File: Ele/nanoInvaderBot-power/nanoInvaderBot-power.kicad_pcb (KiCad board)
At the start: 2 copper layers, 72 x 40 mm, 16 parts, among them J1 S6B-ZR-SM4A-TF(LF)(SN), J2 S6B-ZR-SM4A-TF(LF)(SN), J3 1746142-1, J4 Conn_01x20, P1 USB_C_Plug_USB2.0, U4 BQ25170DSGR, U5 TLV61048DBVT

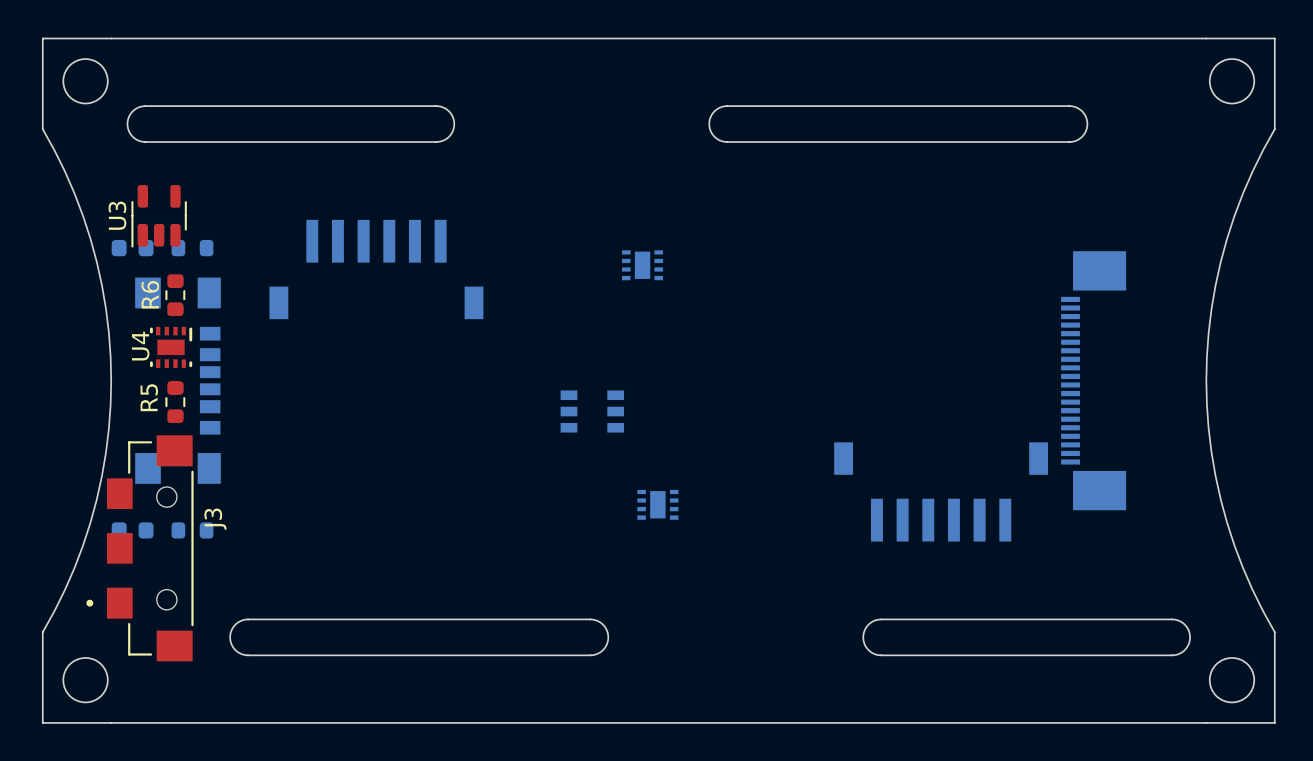
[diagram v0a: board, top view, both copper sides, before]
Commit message: Intermediate state -power layer almost done
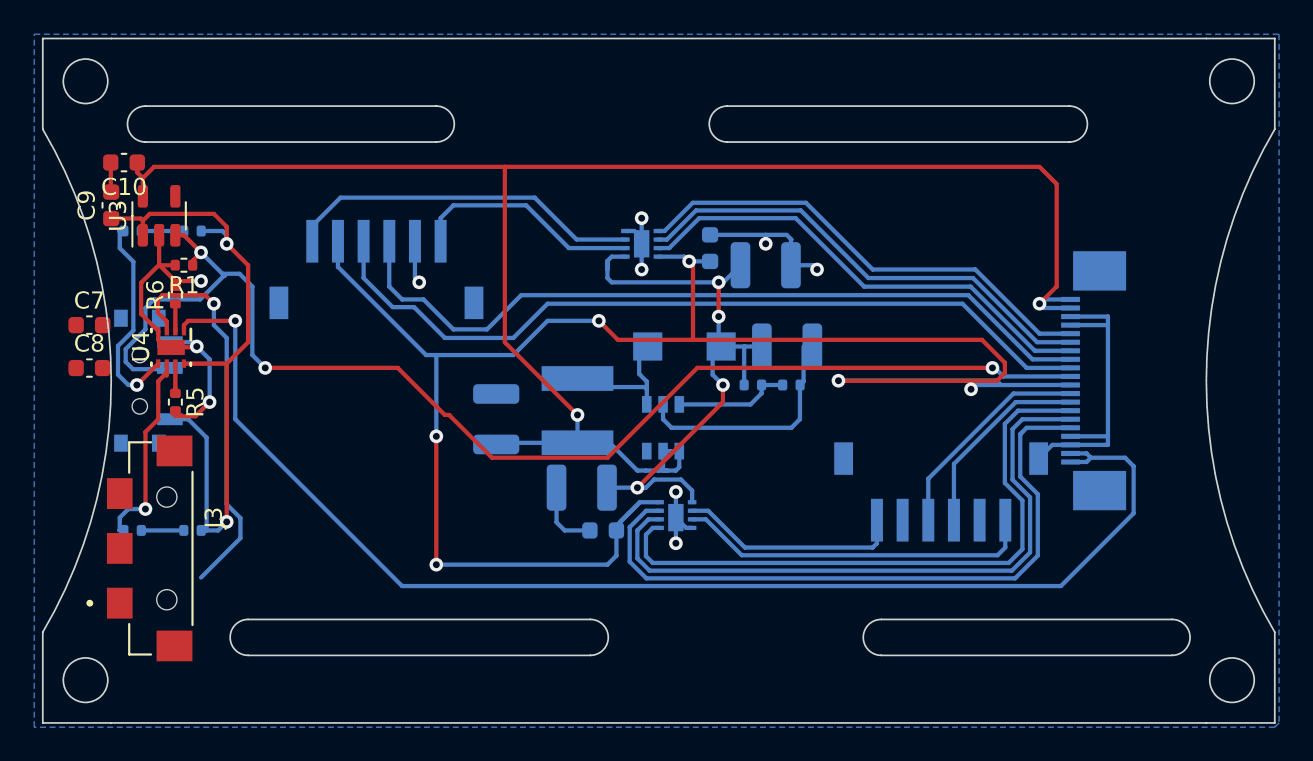
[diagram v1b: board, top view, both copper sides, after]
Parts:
- removed P1: USB_C_Plug_USB2.0, Connector_USB:USB_C_Receptacle_GCT_USB4135-GF-A_6P_TopMnt_Horizontal
- added C1: C, Capacitor_SMD:C_1210_3225Metric, B.Cu at (140.5, 102.2)
- added C10: C, Capacitor_SMD:C_0603_1608Metric, F.Cu at (118.8, 87.2)
- added C2: C, Capacitor_SMD:C_1210_3225Metric, B.Cu at (157.5, 98.0)
- added C3: C, Capacitor_SMD:C_1210_3225Metric, B.Cu at (156.2, 93.2)
- added C4: C, Capacitor_SMD:C_0603_1608Metric, B.Cu at (153.0, 92.2)
- added C5: C, Capacitor_SMD:C_1210_3225Metric, B.Cu at (145.5, 106.2)
- added C6: C, Capacitor_SMD:C_0603_1608Metric, B.Cu at (146.8, 108.8)
- added C7: C, Capacitor_SMD:C_0603_1608Metric, F.Cu at (116.7, 96.8)
- added C8: C, Capacitor_SMD:C_0603_1608Metric, F.Cu at (116.7, 99.3)
- added C9: C, Capacitor_SMD:C_0603_1608Metric, F.Cu at (118.0, 89.8)
- added D3: D, footprints:SDO_B120AF_DIO, B.Cu at (151.5, 98.0)
- added L1: L, footprints:IND_SWPA5040S_SNL, B.Cu at (145.2, 101.8)
- added R1: R, Resistor_SMD:R_0402_1005Metric, F.Cu at (122.2, 93.2)
- added R10: R, Resistor_SMD:R_0402_1005Metric, B.Cu at (155.5, 100.2)
- added R9: R, Resistor_SMD:R_0402_1005Metric, B.Cu at (157.8, 100.2)
- added SW1: SW_SPDT, Button_Switch_SMD:SW_SPDT_PCM12, B.Cu at (120.0, 100.0)
- D1, D2: footprint LED_SMD:LED_0603_1608Metric -> Resistor_SMD:R_0402_1005Metric
- R5, R6, R7, R8: footprint Resistor_SMD:R_0603_1608Metric -> Resistor_SMD:R_0402_1005Metric
- moved U5 4.24 mm to (150.2, 102.8), turned to -90 degrees
- moved U1 1.25 mm to (149.0, 92.0), turned to 0 degrees
- moved U2 1.21 mm to (151.0, 107.8)
- moved D2 1.00 mm to (119.2, 91.2)
- moved R8 1.00 mm to (122.8, 91.2)
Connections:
- J1 pad 3: /MOTOR1_C1 -> /MOTOR1_ENC1
- J1 pad 4: /MOTOR1_C2 -> /MOTOR1_ENC2
- J1 pad SH1: unconnected-(J1-SHIELD-PadSH1) -> /GND
- J1 pad SH2: unconnected-(J1-SHIELD-PadSH1) -> /GND
- J2 pad 3: /MOTOR2_C1 -> /MOTOR2_ENC1
- J2 pad 4: /MOTOR2_C2 -> /MOTOR2_ENC2
- J2 pad SH1: unconnected-(J2-SHIELD-PadSH1) -> /GND
- J2 pad SH2: unconnected-(J2-SHIELD-PadSH1) -> /GND
- J4 pad 1: unconnected-(J4-Pin_1-Pad1) -> /VSYS
- J4 pad 10: unconnected-(J4-Pin_10-Pad10) -> /SYS_EN
- J4 pad 11: unconnected-(J4-Pin_11-Pad11) -> /3V3
- J4 pad 12: unconnected-(J4-Pin_12-Pad12) -> /MOTOR2_ENC1
- J4 pad 13: unconnected-(J4-Pin_13-Pad13) -> /MOTOR2_ENC2
- J4 pad 14: unconnected-(J4-Pin_14-Pad14) -> /MOTOR2_B_MCU
- J4 pad 15: unconnected-(J4-Pin_15-Pad15) -> /MOTOR2_A_MCU
- J4 pad 16: unconnected-(J4-Pin_16-Pad16) -> /MOTOR2_EN_MCU
- J4 pad 17: unconnected-(J4-Pin_17-Pad17) -> /GND
- J4 pad 18: unconnected-(J4-Pin_18-Pad18) -> /GND
- J4 pad 19: unconnected-(J4-Pin_19-Pad19) -> /VUSB
- J4 pad 2: unconnected-(J4-Pin_2-Pad2) -> /VSYS
- J4 pad 20: unconnected-(J4-Pin_20-Pad20) -> /VUSB
- J4 pad 3: unconnected-(J4-Pin_3-Pad3) -> /GND
- J4 pad 4: unconnected-(J4-Pin_4-Pad4) -> /GND
- J4 pad 5: unconnected-(J4-Pin_5-Pad5) -> /MOTOR1_B_MCU
- J4 pad 6: unconnected-(J4-Pin_6-Pad6) -> /MOTOR1_A_MCU
- J4 pad 7: unconnected-(J4-Pin_7-Pad7) -> /MOTOR1_EN_MCU
- J4 pad 8: unconnected-(J4-Pin_8-Pad8) -> /MOTOR1_ENC1
- J4 pad 9: unconnected-(J4-Pin_9-Pad9) -> /MOTOR1_ENC2
- U3 pad 3: /VBATT -> /SYS_EN
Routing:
- net /3V3: track 0.00 -> 107.8 mm, vias 0 -> 6
- net /VSYS: track 0.00 -> 100.2 mm, vias 0 -> 2
- net /GND: track 0.00 -> 78.4 mm, vias 0 -> 10
- net /VUSB: track 0.00 -> 75.5 mm, vias 0 -> 1
- net /SYS_EN: track 0.00 -> 75.4 mm, vias 0 -> 3
- net /MOTOR1_ENC2: track 0.00 -> 47.3 mm
- net /MOTOR1_ENC1: track 0.00 -> 45.9 mm
- net /VBATT: track 0.00 -> 40.1 mm, vias 0 -> 2
- net /MOTOR2_EN_MCU: track 0.00 -> 39.8 mm
- net /MOTOR2_A_MCU: track 0.00 -> 38.2 mm
- net /MOTOR2_B_MCU: track 0.00 -> 36.6 mm
- net /12V: track 0.00 -> 36.2 mm, vias 0 -> 4
- net /MOTOR1_EN_MCU: track 0.00 -> 28.0 mm
- net /MOTOR1_A_MCU: track 0.00 -> 28.0 mm
- net /MOTOR1_B_MCU: track 0.00 -> 28.0 mm
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- added copper zone on B.Cu, net /GND
